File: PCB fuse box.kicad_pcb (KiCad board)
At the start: 2 copper layers, 115.6 x 62 mm, 21 parts, among them J1 6570XX230201_657012230201, J2 6570XX230201_657012230201, J3 436500315, K1 AZ2150-1A-12DEF, K2 AZ2150-1A-12DEF

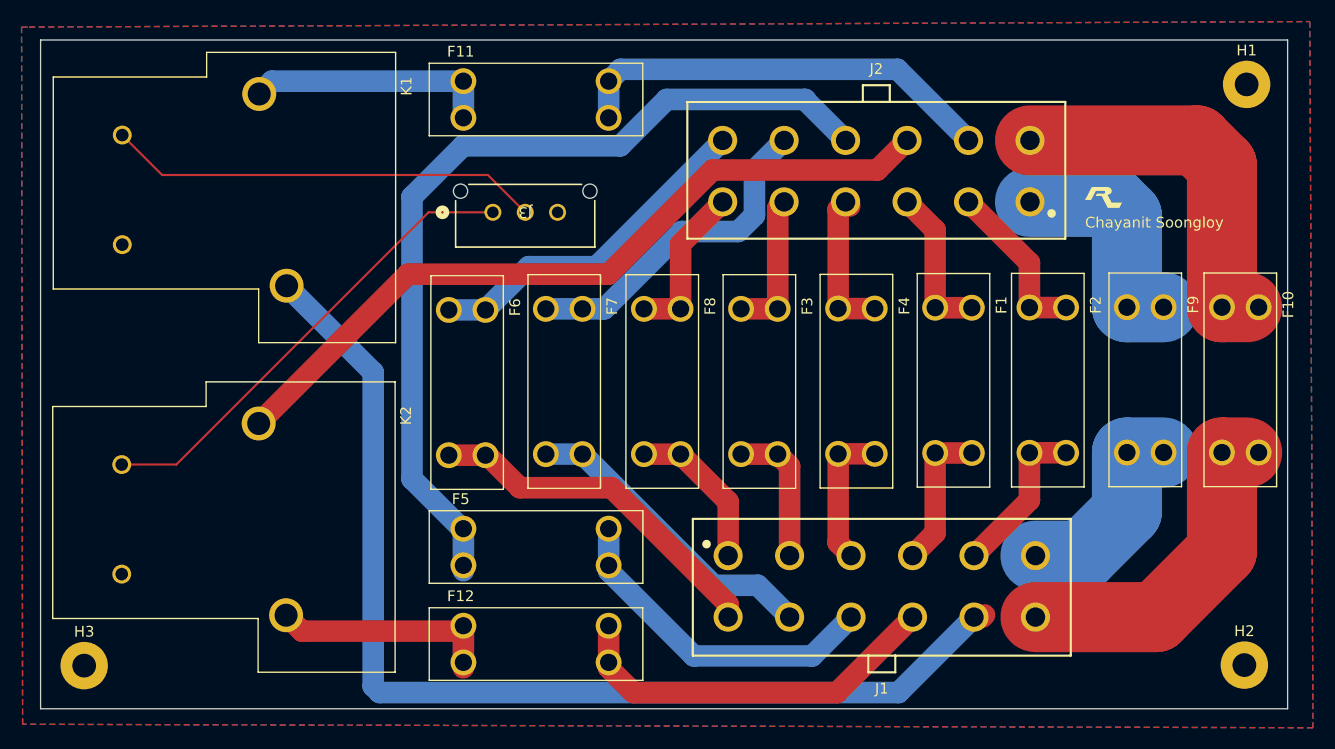
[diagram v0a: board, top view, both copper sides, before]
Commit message: Adjust width
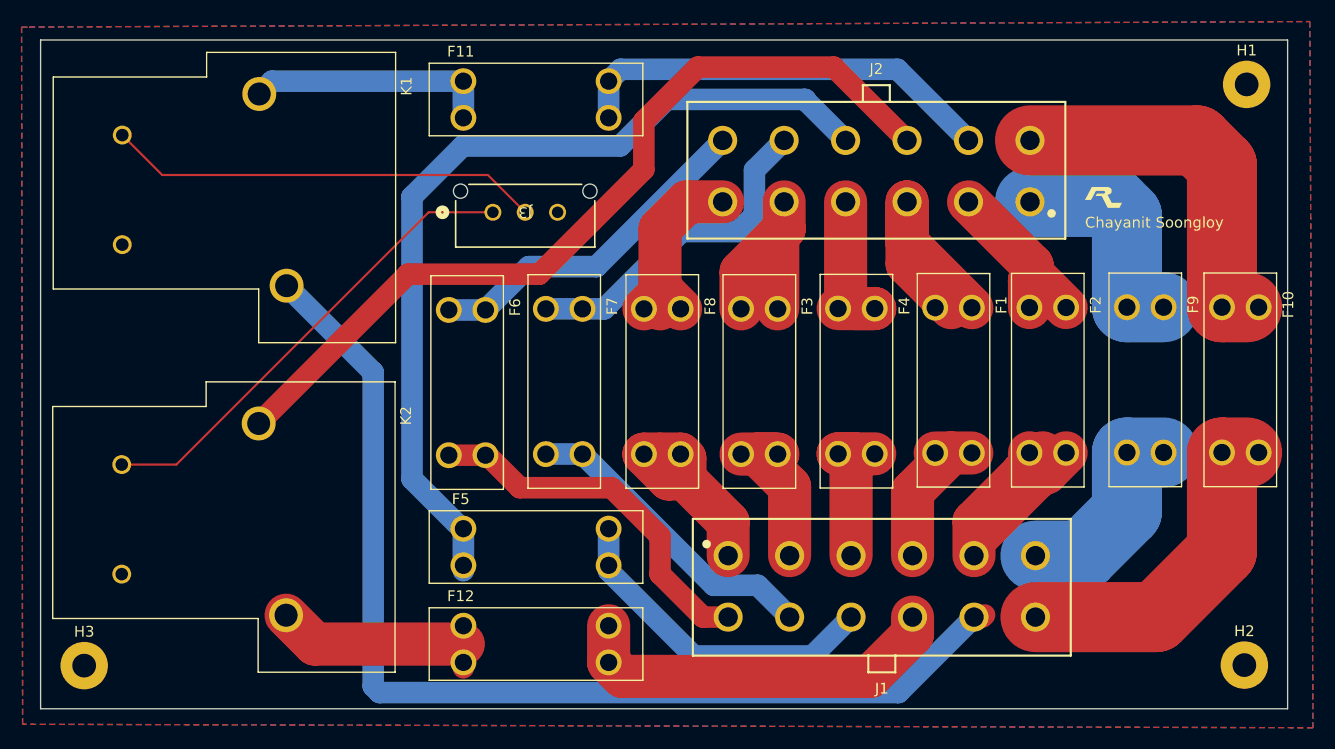
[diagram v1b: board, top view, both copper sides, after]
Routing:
- net 5A: track 15.1 -> 38.1 mm
- net 3: track 14.3 -> 27.2 mm
- net 1A: track 14.6 -> 26.1 mm
- net 6: track 14.9 -> 26.3 mm
- net 5: track 13.6 -> 22.6 mm
- net 2: track 15.5 -> 24.4 mm
- net 9: track 71.0 -> 79.3 mm
- net 4: track 14.1 -> 17.0 mm
- net 2A: track 13.3 -> 16.0 mm
- net 7A: track 32.8 -> 34.2 mm
- net 3A: track 13.3 -> 14.4 mm
- net 4A: track 13.8 -> 14.4 mm
